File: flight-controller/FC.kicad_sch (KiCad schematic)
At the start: 4 parts, among them J2 USB_B_Micro, U2 ESP32-S3-MINI-1, U4 NCP1117ST33T3G

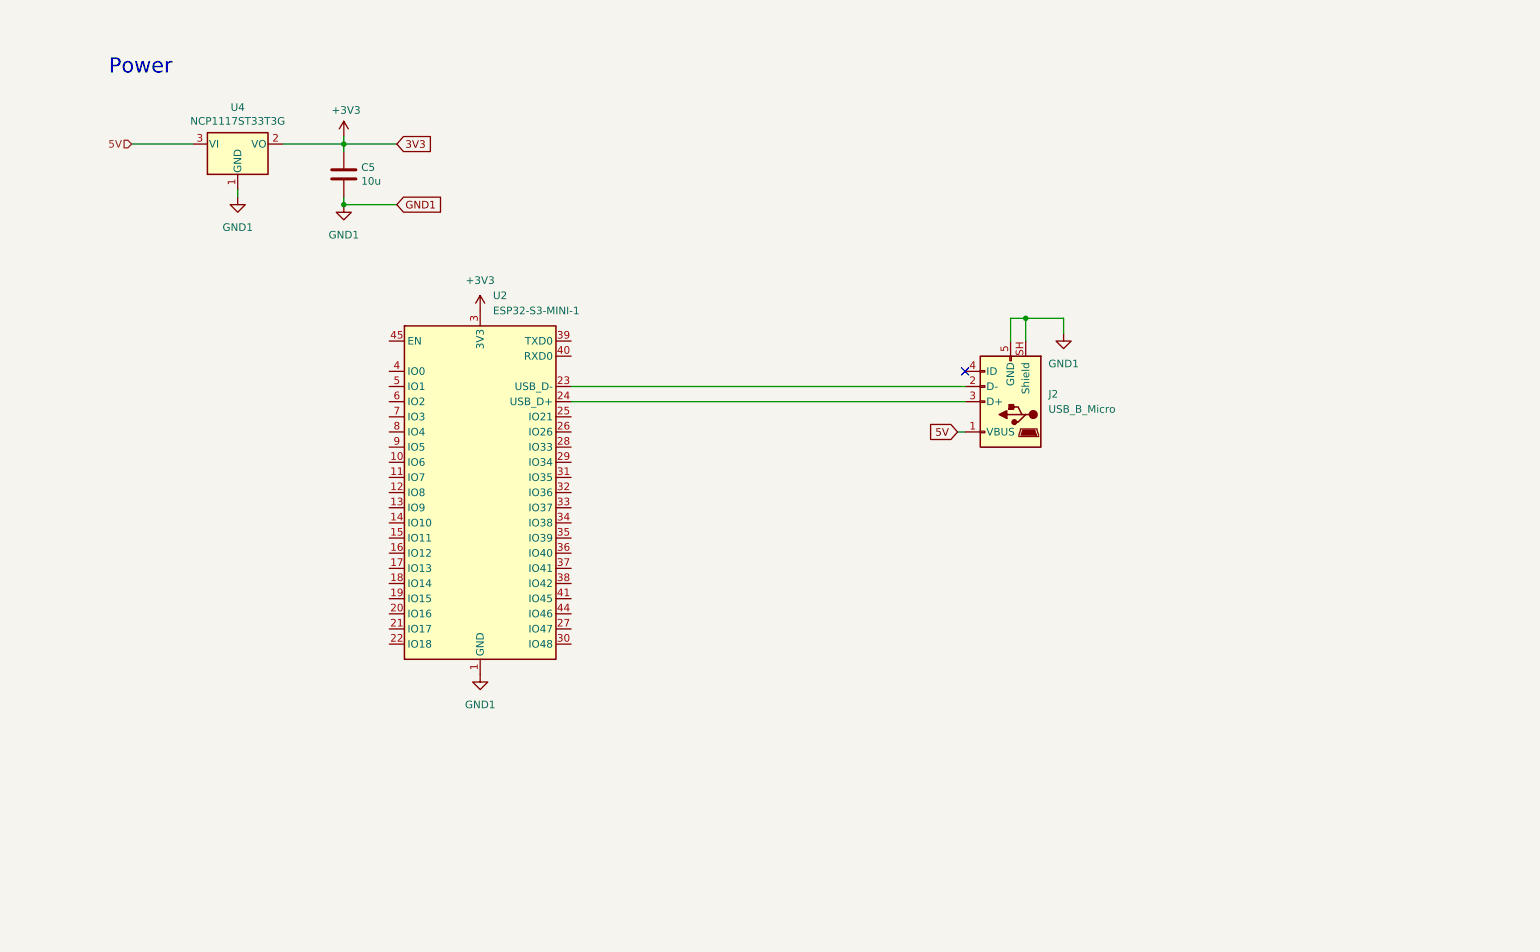
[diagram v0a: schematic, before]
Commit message: sensors
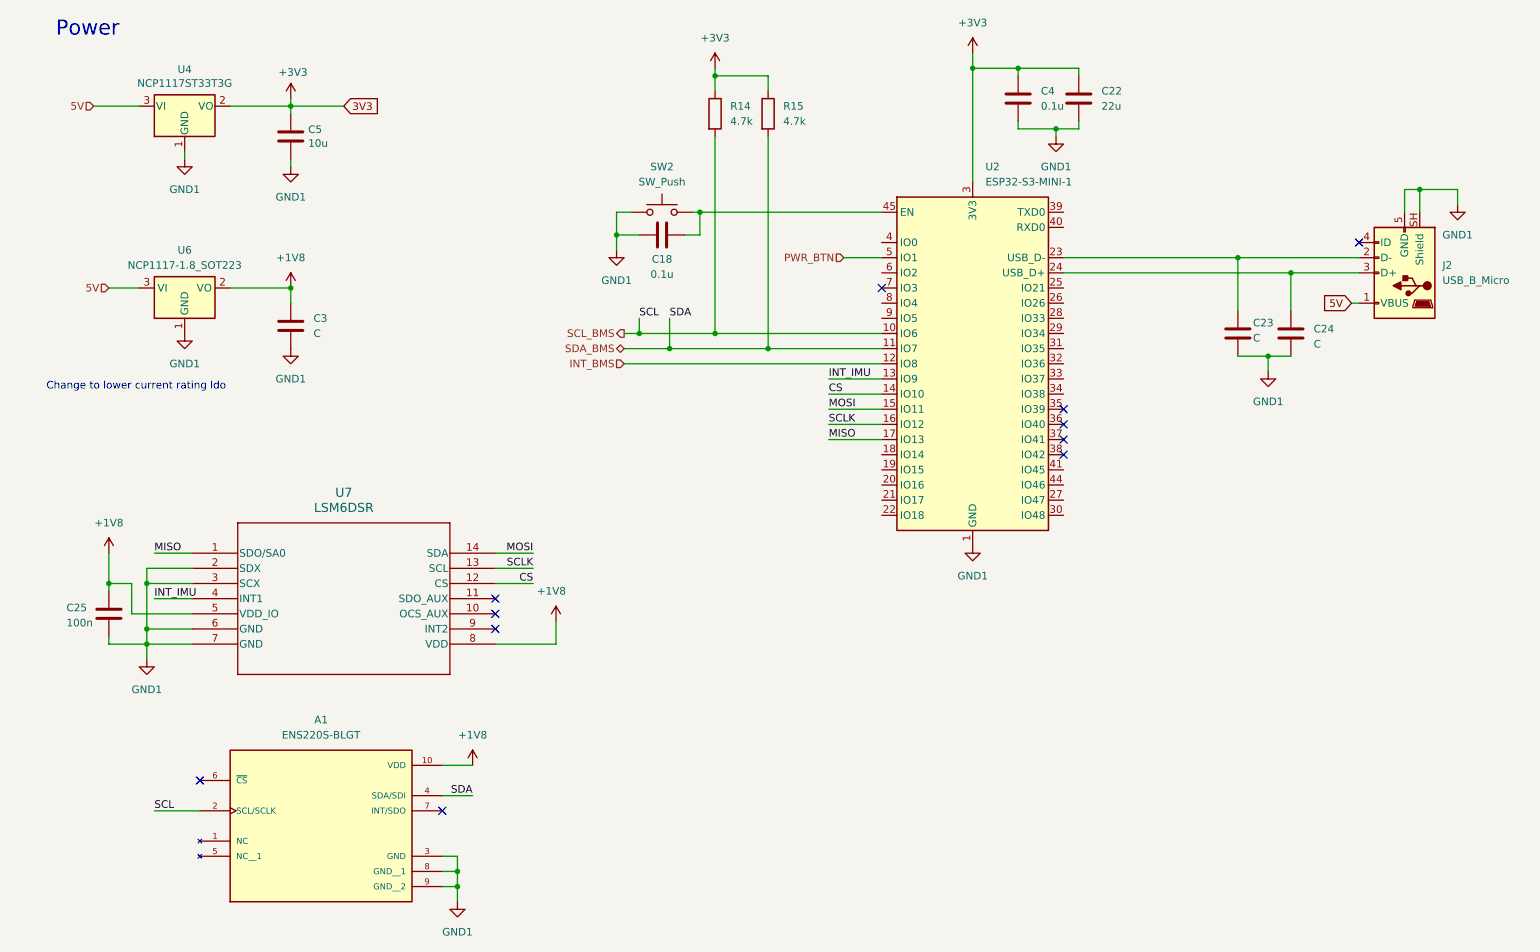
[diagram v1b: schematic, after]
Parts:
- added A1: ENS220S-BLGT, ENS220S-BLGT:XDCR_ENS220S-BLGT, symbol ENS220S-BLGT:ENS220S-BLGT
- added C18, C4: 0.1u, symbol Device:C
- added C22: 22u, symbol Device:C
- added C23, C24, C3: C, symbol Device:C
- added C25: 100n, symbol Device:C
- added R14, R15: 4.7k, symbol Device:R
- added SW2: SW_Push, symbol Switch:SW_Push
- added U6: NCP1117-1.8_SOT223, Package_TO_SOT_SMD:SOT-223-3_TabPin2, symbol Regulator_Linear:NCP1117-1.8_SOT223
- added U7: LSM6DSR, LGA_M6DSR_STM, symbol 2026-04-10_00-11-54:LSM6DSR
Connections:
- net +3V3: now also C22.1, C4.1, R14.1, R15.1
- net 5V: now also U6.3 (VI)
- net GND1: now also A1.3 (GND), A1.8 (GND__1), A1.9 (GND__2), C18.1, C22.2, C23.2, C24.2, C25.2, C3.2, C4.2, SW2.1, U6.1 (GND), U7.2 (SDX), U7.3 (SCX), U7.6 (GND), U7.7 (GND)
- net at J2.2 (D-), U2.23 (USB_D-): now also C23.1
- net at J2.3 (D+), U2.24 (USB_D+): now also C24.1
- net SCL_BMS: now reaches U2.10 (IO6)
- net SCL_BMS: now also A1.2 (SCL/SCLK), R14.2
- net SDA_BMS: now reaches U2.11 (IO7)
- net SDA_BMS: now also A1.4 (SDA/SDI), R15.2
- net INT_BMS: now reaches U2.12 (IO8)
- net INT_IMU: now reaches U2.13 (IO9)
- net INT_IMU: now also U7.4 (INT1)
- net CS: now reaches U2.14 (IO10)
- net CS: now also U7.12 (CS)
- net MOSI: now reaches U2.15 (IO11)
- net MOSI: now also U7.14 (SDA)
- net SCLK: now reaches U2.16 (IO12)
- net SCLK: now also U7.13 (SCL)
- net MISO: now reaches U2.17 (IO13)
- net MISO: now also U7.1 (SDO/SA0)
- net at U2.45 (EN): now also C18.2, SW2.2
- net PWR_BTN: now reaches U2.5 (IO1)
- new net +1V8: A1.10 (VDD), C25.1, C3.1, U6.2 (VO), U7.5 (VDD_IO), U7.8 (VDD)
- no-connect marks 1 -> 11
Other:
- note added: "Change to lower current rating ldo"
- moved on the sheet: C5, J2, U2, U4
